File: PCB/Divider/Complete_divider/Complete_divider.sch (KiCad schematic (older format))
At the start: 0 parts

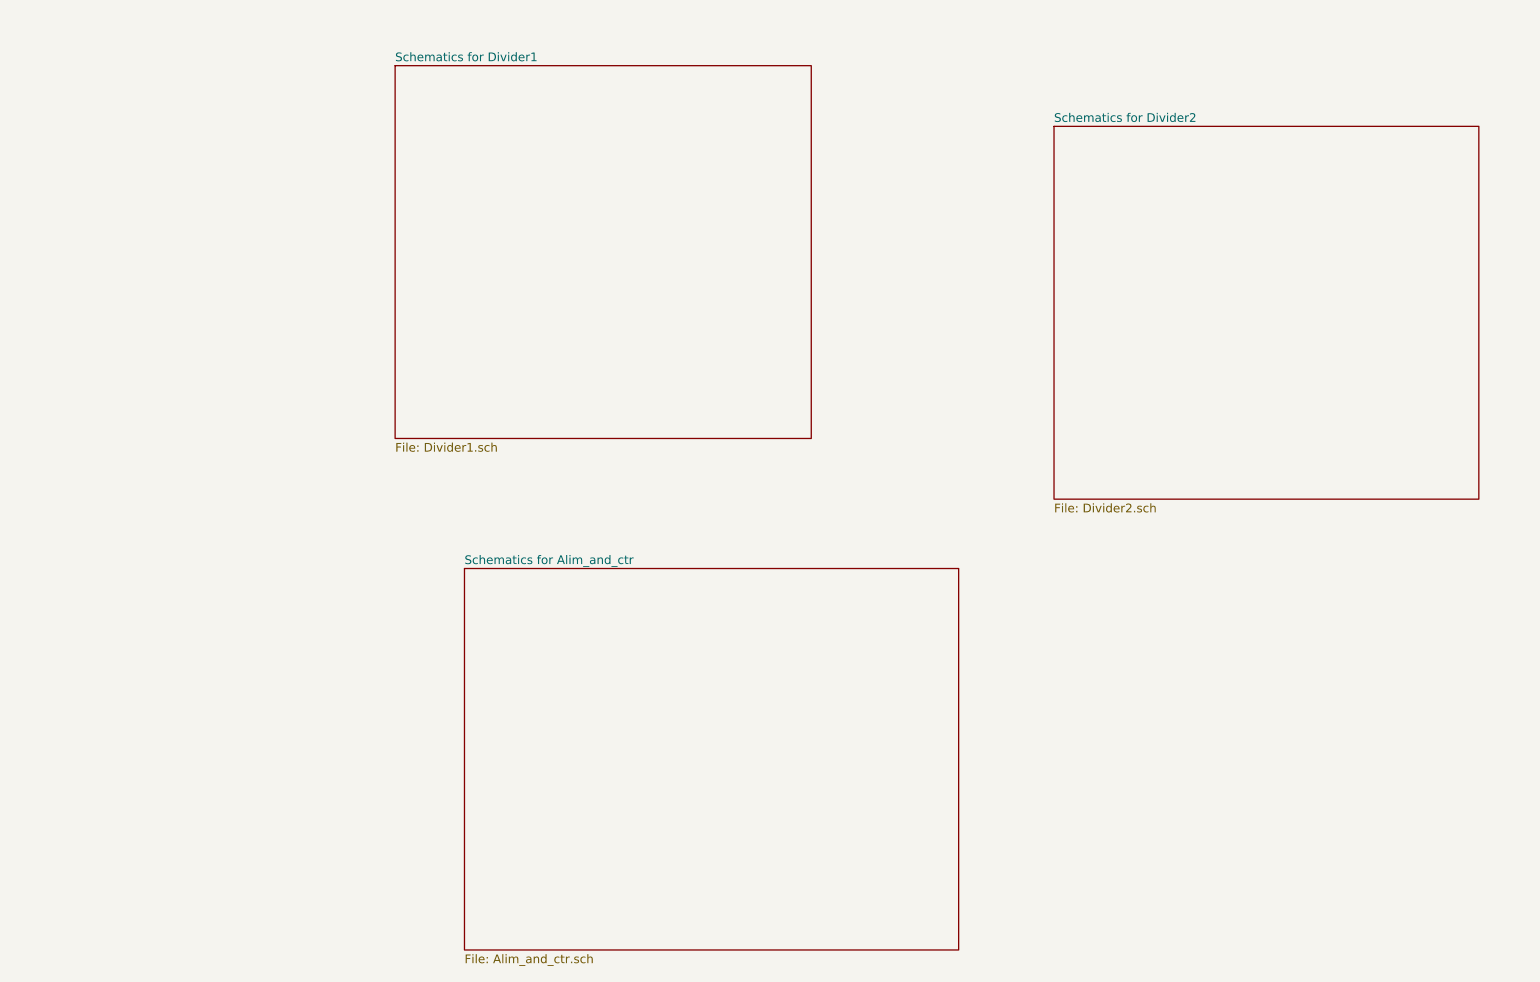
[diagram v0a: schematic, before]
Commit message: Small modifications
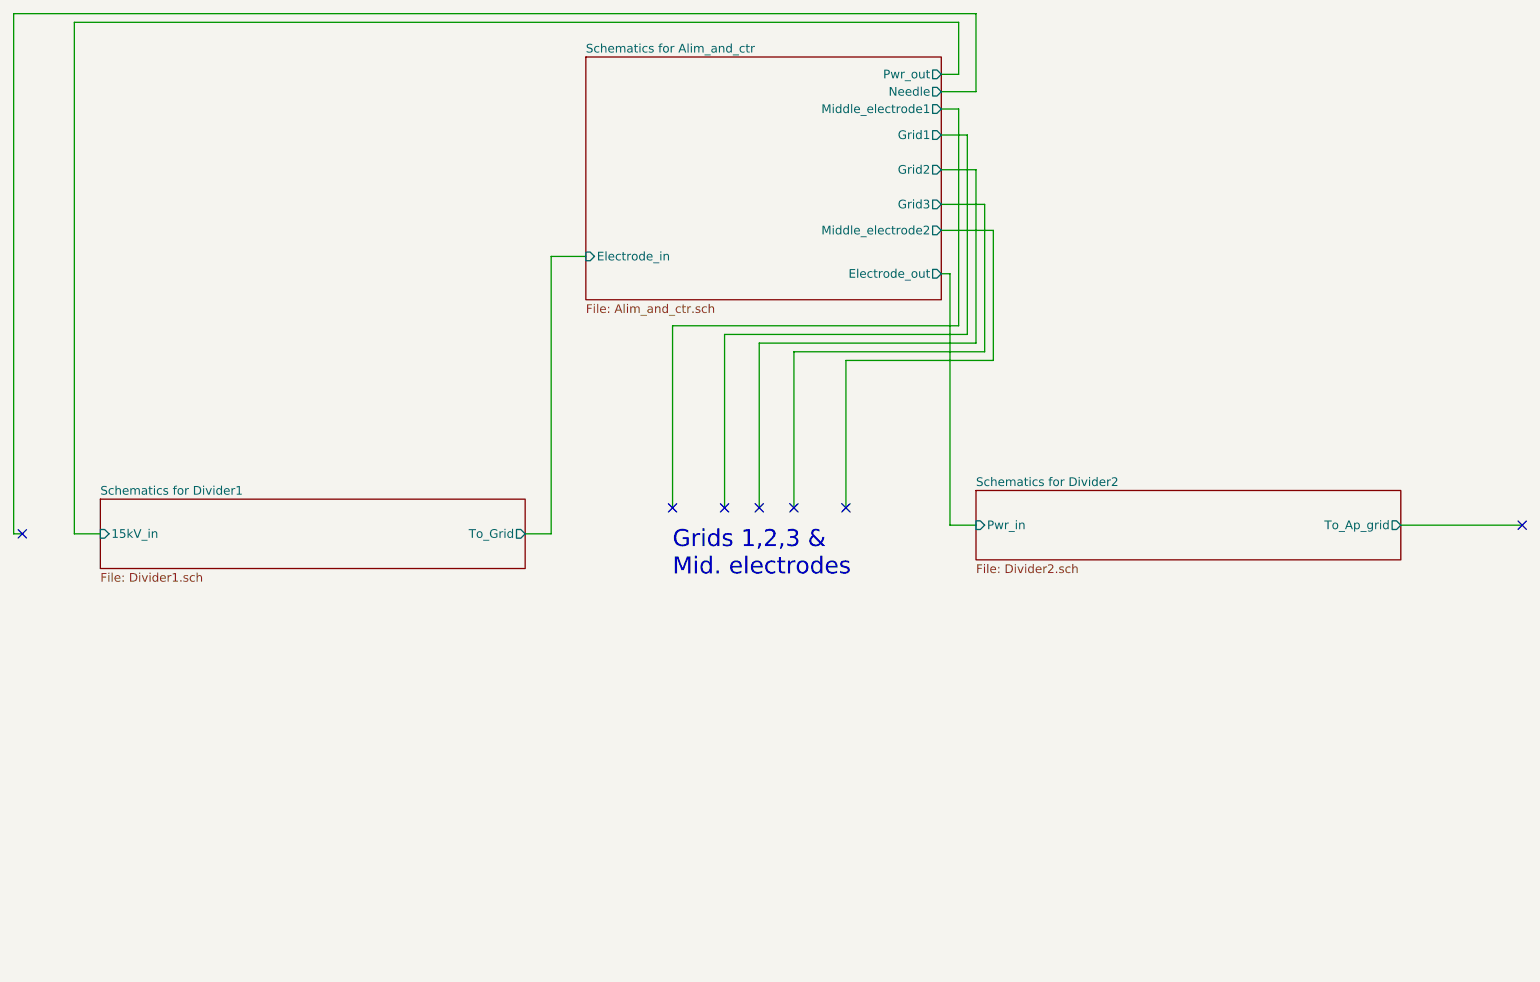
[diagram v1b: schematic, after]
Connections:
- no-connect marks 0 -> 7
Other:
- note added: "Grids 1,2,3 &\nMid. electrodes\n"
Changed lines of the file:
@@
 $EndDescr
 $Sheet
-S 3250 4350 2850 2200
+S 6200 3900 2450 400
+U 5E63EFA9
+F0 "Schematics for Divider2" 50
+F1 "Divider2.sch" 50
+F2 "Pwr_in" I L 6200 4100 50
+F3 "To_Ap_grid" O R 8650 4100 50
+$EndSheet
+Wire Wire Line
+	3600 4150 3750 4150
+Wire Wire Line
+	3750 4150 3750 2550
+Wire Wire Line
+	3750 2550 3950 2550
+Wire Wire Line
+	4750 3000 6150 3000
+Wire Wire Line
+	6150 3000 6150 1850
+Wire Wire Line
+	6150 1850 6000 1850
+Wire Wire Line
+	4750 3000 4750 4000
+Wire Wire Line
+	4950 3050 6200 3050
+Wire Wire Line
+	6200 2050 6000 2050
+Wire Wire Line
+	5150 3100 6250 3100
+Wire Wire Line
+	6250 2250 6000 2250
+Wire Wire Line
+	6000 2650 6050 2650
+Wire Wire Line
+	6050 4100 6200 4100
+$Sheet
+S 1150 3950 2450 400
+U 5E6FA86A
+F0 "Schematics for Divider1" 50
+F1 "Divider1.sch" 50
+F2 "15kV_in" I L 1150 4150 50
+F3 "To_Grid" O R 3600 4150 50
+$EndSheet
+Wire Wire Line
+	6000 1500 6100 1500
+Wire Wire Line
+	6100 1500 6100 1200
+Wire Wire Line
+	6100 1200 1000 1200
+Wire Wire Line
+	1000 1200 1000 4150
+Wire Wire Line
+	1000 4150 1150 4150
+NoConn ~ 5150 4000
+NoConn ~ 4950 4000
+NoConn ~ 4750 4000
+Text Notes 4450 4400 0    98   ~ 0
+Grids 1,2,3 &\nMid. electrodes\n
+$Sheet
+S 3950 1400 2050 1400
 U 5E63F098
 F0 "Schematics for Alim_and_ctr" 50
 F1 "Alim_and_ctr.sch" 50
+F2 "Grid1" O R 6000 1850 50
+F3 "Grid2" O R 6000 2050 50
+F4 "Grid3" O R 6000 2250 50
+F5 "Electrode_in" I L 3950 2550 50
+F6 "Electrode_out" O R 6000 2650 50
+F7 "Pwr_out" O R 6000 1500 50
+F8 "Middle_electrode1" O R 6000 1700 50
+F9 "Middle_electrode2" O R 6000 2400 50
+F10 "Needle" O R 6000 1600 50
 $EndSheet
-$Sheet
-S 2850 1450 2400 2150
-U 5E6FA86A
-F0 "Schematics for Divider1" 50
-F1 "Divider1.sch" 50
-$EndSheet
-$Sheet
-S 6650 1800 2450 2150
-U 5E63EFA9
-F0 "Schematics for Divider2" 50
-F1 "Divider2.sch" 50
-$EndSheet
+Wire Wire Line
+	6300 3150 5450 3150
+Wire Wire Line
+	6000 2400 6300 2400
+Wire Wire Line
+	6200 2050 6200 3050
+Wire Wire Line
+	6300 2400 6300 3150
+Wire Wire Line
+	6250 3100 6250 2250
+Wire Wire Line
+	4450 4000 4450 2950
+Wire Wire Line
+	4450 2950 6100 2950
+Wire Wire Line
+	6100 2950 6100 1700
+Wire Wire Line
+	6100 1700 6000 1700
+NoConn ~ 4450 4000
+NoConn ~ 5450 4000
+Wire Wire Line
+	4950 4000 4950 3050
+Wire Wire Line
+	5150 4000 5150 3100
+Wire Wire Line
+	5450 4000 5450 3150
+Wire Wire Line
+	6050 2650 6050 4100
+NoConn ~ 9350 4100
+Wire Wire Line
+	8650 4100 9350 4100
+Wire Wire Line
+	6000 1600 6200 1600
+Wire Wire Line
+	6200 1600 6200 1150
+Wire Wire Line
+	6200 1150 650  1150
+Wire Wire Line
+	650  1150 650  4150
+Wire Wire Line
+	650  4150 700  4150
+NoConn ~ 700  4150
 $EndSCHEMATC
